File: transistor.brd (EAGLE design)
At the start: 17.8 x 29.2 mm, 4 parts, among them T1 BC547N

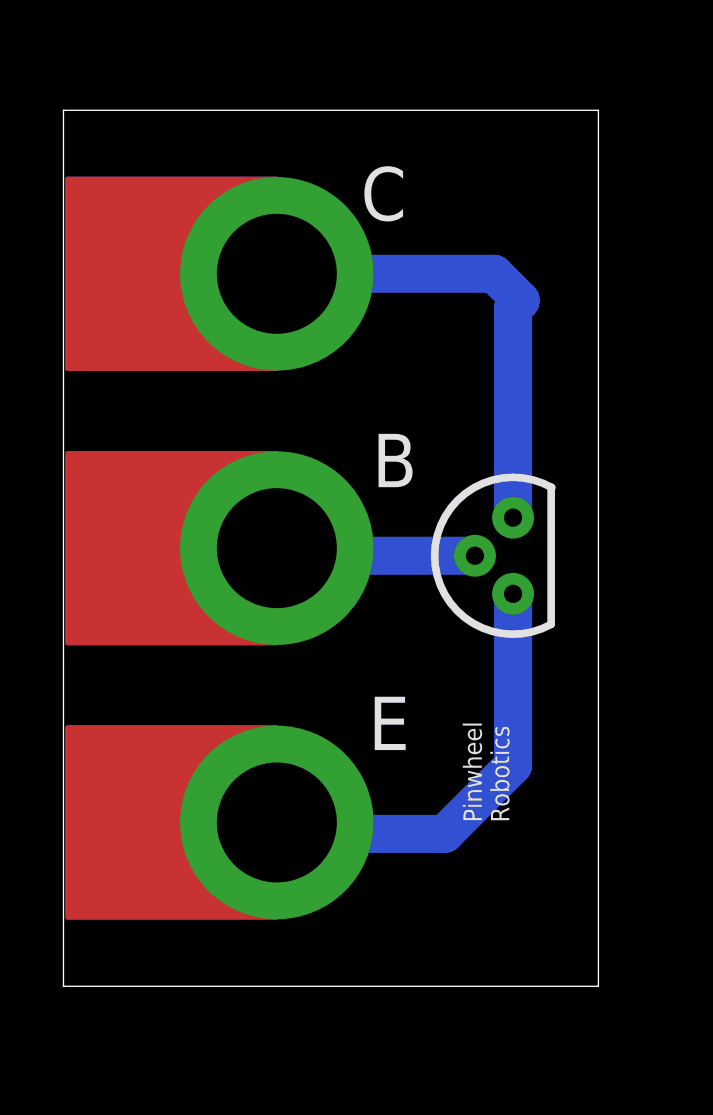
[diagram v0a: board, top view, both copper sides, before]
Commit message: updte
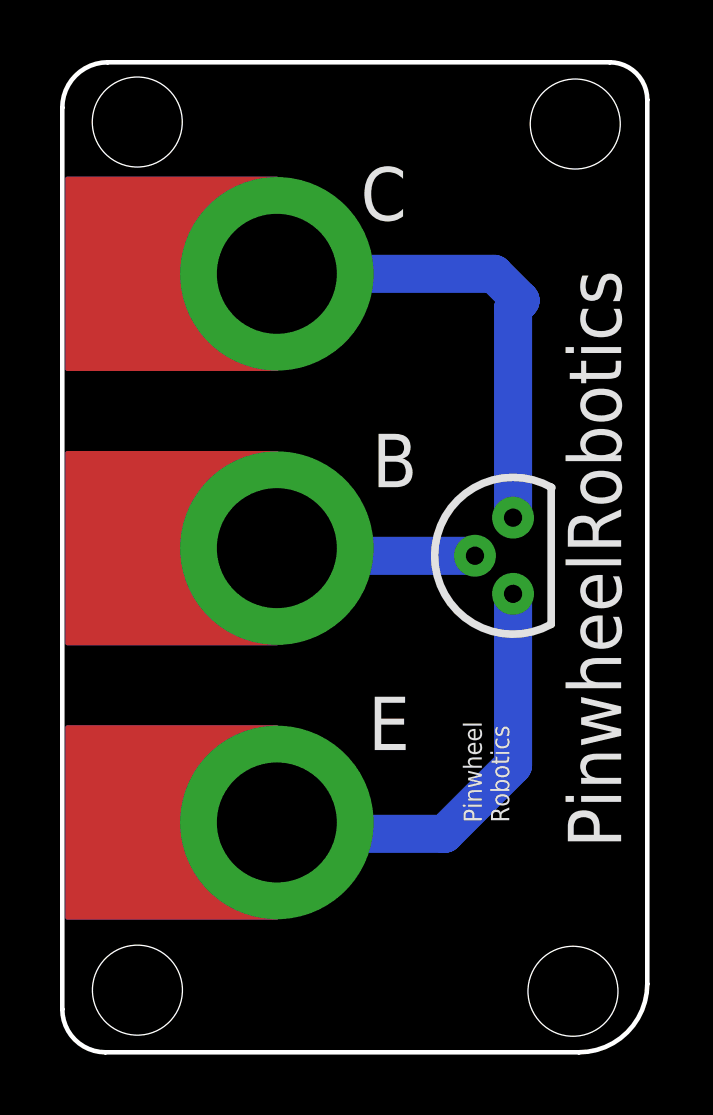
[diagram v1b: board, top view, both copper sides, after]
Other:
- board size 17.8 x 29.2 mm -> 19.5 x 33 mm
- board text added: "PinwheelRobotics"
- board text added: "care@pinwheel"
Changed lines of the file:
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@@
 <drawing>
 <settings>
-<setting alwaysvectorfont="no"/>
+<setting alwaysvectorfont="yes"/>
 <setting verticaltext="up"/>
 </settings>
-<grid distance="50" unitdist="mil" unit="mm" style="lines" multiple="1" display="yes" altdistance="5" altunitdist="mil" altunit="mm"/>
+<grid distance="0.5" unitdist="mm" unit="mm" style="lines" multiple="1" display="yes" altdistance="0.003125" altunitdist="mic" altunit="mm"/>
 <layers>
 <layer number="1" name="Top" color="4" fill="1" visible="yes" active="yes"/>
@@
 <layer number="43" name="vRestrict" color="2" fill="10" visible="yes" active="yes"/>
 <layer number="44" name="Drills" color="7" fill="1" visible="no" active="yes"/>
-<layer number="45" name="Holes" color="7" fill="1" visible="no" active="yes"/>
+<layer number="45" name="Holes" color="7" fill="1" visible="yes" active="yes"/>
 <layer number="46" name="Milling" color="3" fill="1" visible="no" active="yes"/>
 <layer number="47" name="Measures" color="7" fill="1" visible="no" active="yes"/>
@@
 <board>
 <plain>
-<wire x1="2.54" y1="12.7" x2="20.371" y2="12.7" width="0" layer="20"/>
-<wire x1="20.371" y1="12.7" x2="20.371" y2="41.9" width="0" layer="20"/>
-<wire x1="20.371" y1="41.9" x2="2.54" y2="41.9" width="0" layer="20"/>
-<wire x1="2.54" y1="41.9" x2="2.54" y2="12.7" width="0" layer="20"/>
 <text x="12.7" y="20.574" size="1.778" layer="21">E</text>
 <text x="12.827" y="29.337" size="1.778" layer="21">B</text>
@@
 <text x="17.399" y="18.161" size="0.6096" layer="21" rot="R90">Pinwheel
 Robotics</text>
+<hole x="4.999659375" y="41.508721875" drill="3"/>
+<hole x="19.599125" y="41.442590625" drill="3"/>
+<hole x="19.5227625" y="12.5339" drill="3"/>
+<hole x="5.004790625" y="12.57065625" drill="3"/>
+<wire x1="2.5" y1="41.986021875" x2="2.5" y2="11.936315625" width="0.1524" layer="20"/>
+<wire x1="2.5" y1="11.936315625" x2="3.936315625" y2="10.5" width="0.1524" layer="20" curve="90"/>
+<wire x1="3.936315625" y1="10.5" x2="19.722221875" y2="10.5" width="0.1524" layer="20"/>
+<wire x1="19.722221875" y1="10.5" x2="22" y2="12.777778125" width="0.1524" layer="20" curve="90"/>
+<wire x1="22" y1="12.777778125" x2="22" y2="42.24761875" width="0.1524" layer="20"/>
+<wire x1="22" y1="42.24761875" x2="20.74761875" y2="43.5" width="0.1524" layer="20" curve="90"/>
+<wire x1="20.74761875" y1="43.5" x2="4.013978125" y2="43.5" width="0.1524" layer="20"/>
+<wire x1="4.013978125" y1="43.5" x2="2.5" y2="41.986021875" width="0.1524" layer="20" curve="90"/>
+<text x="21.128425" y="17.31673125" size="1.778" layer="21" rot="R90">PinwheelRobotics</text>
+<text x="19.48631875" y="36.38705625" size="1.778" layer="22" rot="MR270">care@pinwheel</text>
 </plain>
 <attributes>
